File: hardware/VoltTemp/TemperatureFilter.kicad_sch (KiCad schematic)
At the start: 7 parts, among them U7 Opamp_Dual

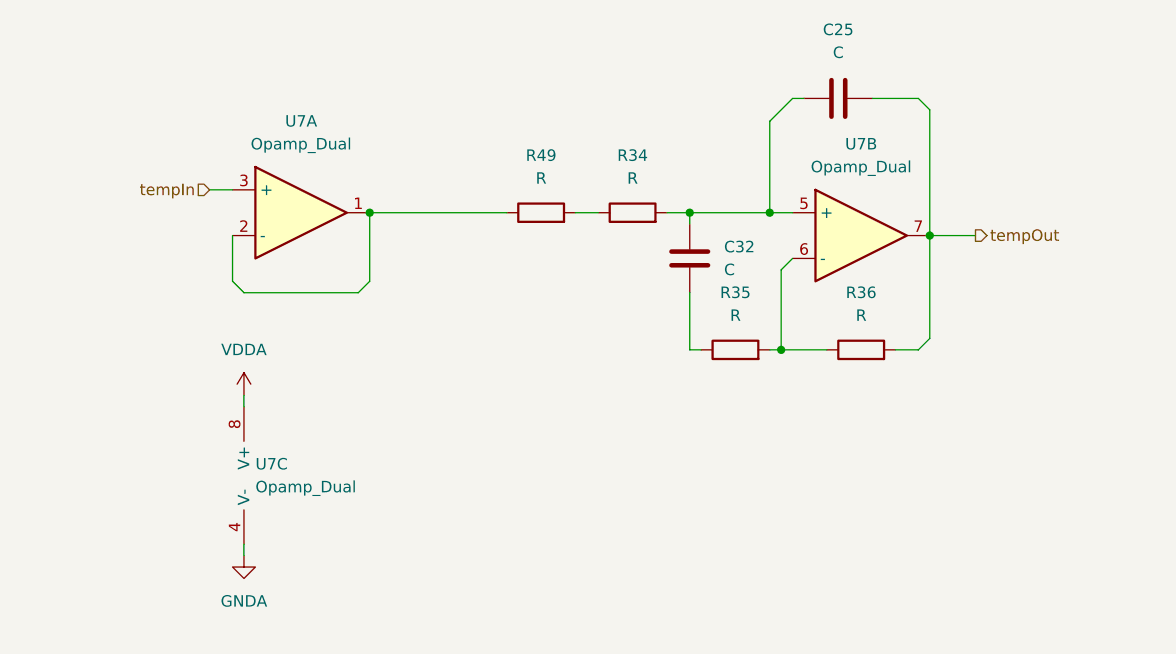
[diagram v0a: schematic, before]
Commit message: schematic mostly done
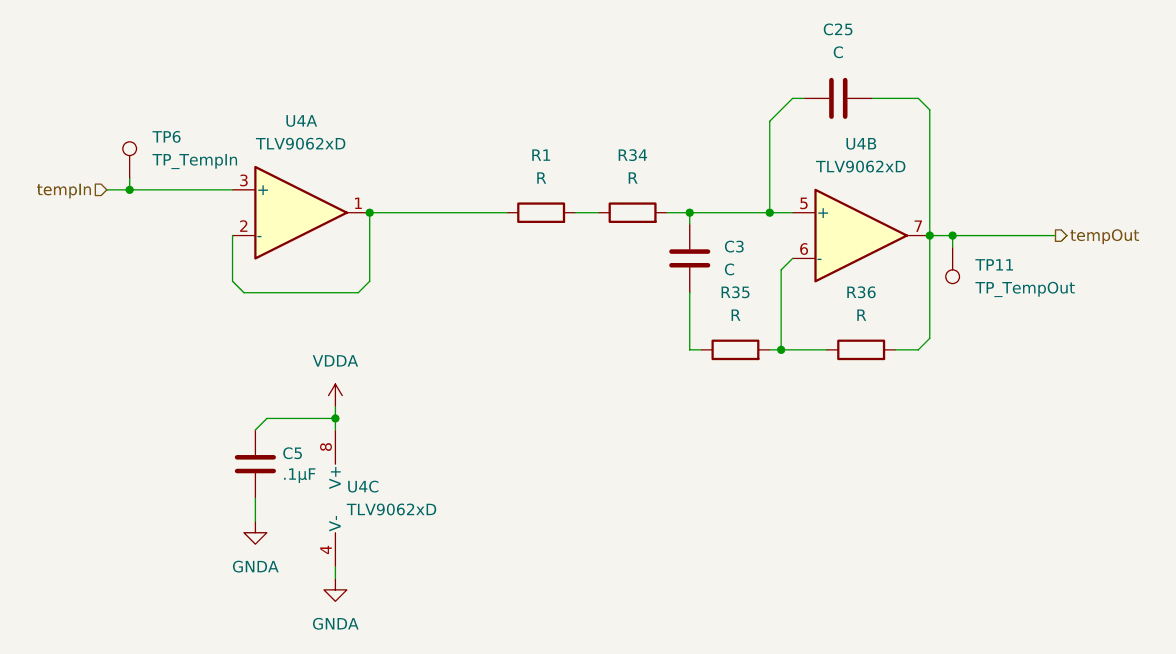
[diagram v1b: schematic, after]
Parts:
- removed U7: Opamp_Dual, symbol Device:Opamp_Dual
- added C5: .1μF, Capacitor_SMD:C_0603_1608Metric_Pad1.08x0.95mm_HandSolder, symbol Device:C
- added TP11: TP_TempOut, TestPoint:TestPoint_Pad_1.0x1.0mm, symbol Connector:TestPoint
- added TP6: TP_TempIn, TestPoint:TestPoint_Pad_1.0x1.0mm, symbol Connector:TestPoint
- added U4: TLV9062xD, Package_SO:SOIC-8_3.9x4.9mm_P1.27mm, symbol Amplifier_Operational:TLV9062xD
- C25: footprint (none) -> Capacitor_SMD:C_0805_2012Metric_Pad1.18x1.45mm_HandSolder
- C3: renamed from C32; footprint (none) -> Capacitor_SMD:C_0805_2012Metric_Pad1.18x1.45mm_HandSolder
- R1: renamed from R49; footprint (none) -> Resistor_SMD:R_0603_1608Metric_Pad0.98x0.95mm_HandSolder
- R34, R35, R36: footprint (none) -> Resistor_SMD:R_0603_1608Metric_Pad0.98x0.95mm_HandSolder
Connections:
- net GNDA: now also C5.2, U4.4 (V-)
- net VDDA: now also C5.1, U4.8 (V+)
- net tempIn: now also TP6.1, U4.3 (+)
- net tempOut: now also TP11.1, U4.7
- net at C25.1, C3.1, R34.2: now also U4.5 (+)
- net at R35.2, R36.1: now also U4.6 (-)
- net at R1.1: now also U4.1, U4.2 (-)
